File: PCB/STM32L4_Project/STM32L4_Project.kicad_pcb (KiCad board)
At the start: 2 copper layers, 37 parts, among them J1 USB_B_Micro, J2 Conn_01x07_Male, J3 Conn_01x03_Female, J4 ARM 10pin, U1 XC6206P332MR, U2 LM386, U3 USBLC6-2SC6, U4 STM32L432KBU6

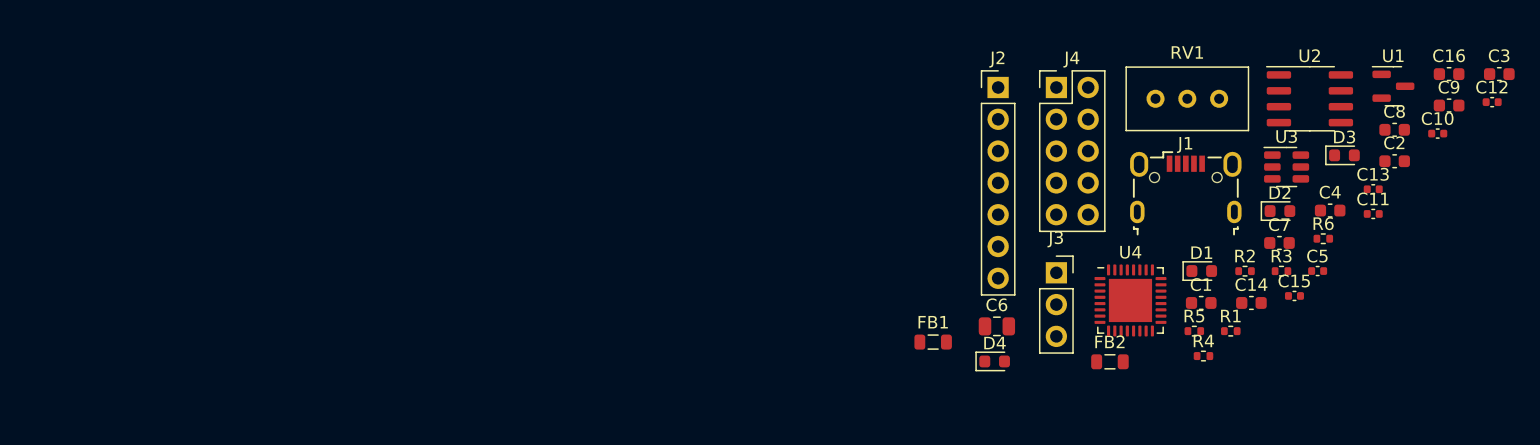
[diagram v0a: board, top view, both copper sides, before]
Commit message: More work on PCB
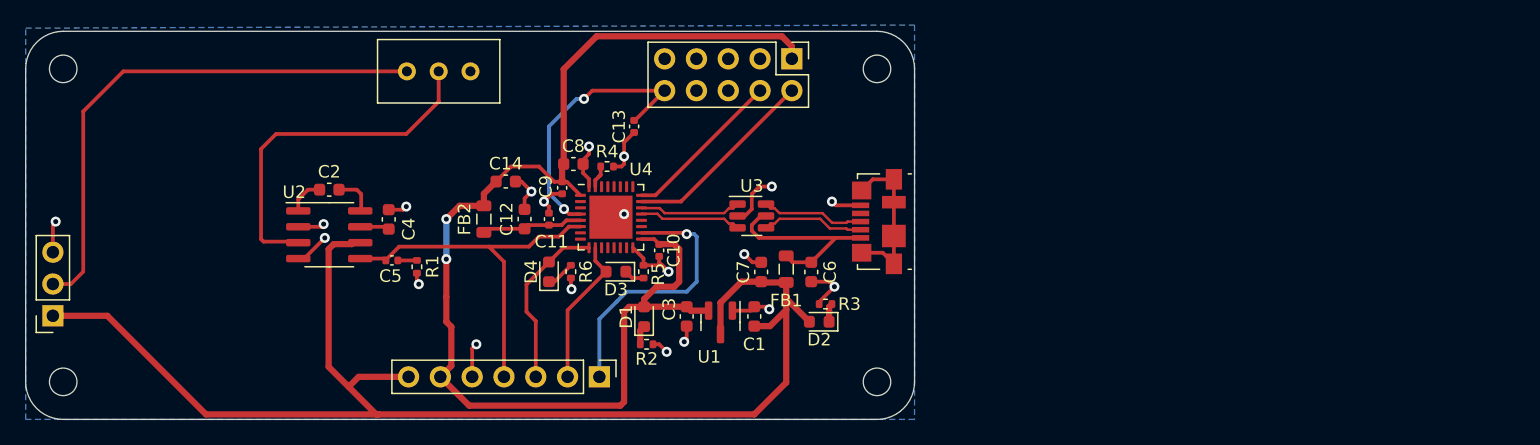
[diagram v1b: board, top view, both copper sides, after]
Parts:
- removed the C12 at (169.1, 42.7)
- removed the C6 at (129.6, 60.6)
- added H1: MountingHole, MountingHole:MountingHole_2.2mm_M2, F.Cu at (120.0, 40.0)
- added H2: MountingHole, MountingHole:MountingHole_2.2mm_M2, F.Cu at (120.0, 65.0)
- added H3: MountingHole, MountingHole:MountingHole_2.2mm_M2, F.Cu at (55.0, 65.0)
- added H4: MountingHole, MountingHole:MountingHole_2.2mm_M2, F.Cu at (55.0, 40.0)
- C5: value 0.1u -> 10pF
- J1: footprint Connector_USB:USB_Micro-B_Wuerth_629105150521 -> Connector_USB:USB_Micro-B_Molex_47346-0001
- R1: value 10k -> 100
- moved C2 85.1 mm to (76.2, 49.6)
- moved J3 80.2 mm to (54.2, 59.7), turned to 180 degrees
- moved U2 79.1 mm to (76.2, 53.2)
- moved C14 75.8 mm to (90.3, 49.0)
- moved C4 75.2 mm to (81.0, 52.0), turned to 90 degrees
- moved C5 74.0 mm to (81.2, 55.3), turned to 180 degrees
- moved C8 70.1 mm to (95.8, 47.6)
- moved C9 70.1 mm to (94.8, 49.5), turned to -90 degrees
- moved C3 67.7 mm to (104.8, 59.8), turned to -90 degrees
- moved C11 65.9 mm to (93.8, 52.0), turned to 90 degrees
- moved R1 65.2 mm to (83.2, 55.8), turned to 90 degrees
- moved RV1 64.9 mm to (82.5, 40.2), turned to 180 degrees
- moved R6 60.2 mm to (95.5, 56.2), turned to 90 degrees
- moved D3 58.9 mm to (99.2, 56.2), turned to 180 degrees
- moved C12 58.4 mm to (91.8, 52.0), turned to 90 degrees
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- renumbered C11 to C10, C13 to C11, C14 to C12, C15 to C13, C16 to C14, C7 to C6, C8 to C7, C9 to C8, C10 to C9
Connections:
- C5 pad 2: Net-(C5-Pad2) -> ADC_IN
- J2 pad 1: PA3 -> PA8
- J2 pad 3: PA8 -> PA3
- J2 pad 5: +5V -> GND
- J2 pad 7: GND -> +5V
- U2 pad 5: Net-(C5-Pad2) -> ADC_IN
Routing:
- net +5V: track 0.00 -> 107.9 mm
- net +3V3: track 0.00 -> 96.7 mm, vias 0 -> 2
- net GND: track 0.00 -> 51.8 mm, vias 0 -> 20
- net RADAR_OUT: track 0.00 -> 42.8 mm
- net ADC_IN: track 0.00 -> 29.7 mm
- net Net-(RV1-Pad2): track 0.00 -> 28.5 mm
- net NRST: track 0.00 -> 22.4 mm, vias 0 -> 2
- net PA8: track 0.00 -> 21.8 mm, vias 0 -> 1
- net VBUS: track 0.00 -> 15.8 mm
- net SWDIO: track 0.00 -> 15.7 mm
- net PA3: track 0.00 -> 13.9 mm
- net SWCLCK: track 0.00 -> 12.9 mm
- net unconnected-(J1-Pad6): track 0.00 -> 12.6 mm
- net PA4: track 0.00 -> 11.9 mm
- net USB_CONN_D+: track 0.00 -> 8.22 mm
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- added copper zone on B.Cu, net GND
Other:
- board outline added: 71 x 31 mm
